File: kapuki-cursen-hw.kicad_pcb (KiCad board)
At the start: 2 copper layers, 27 parts, among them J1 Conn_01x02, J2 Conn_01x02, J3 Conn_01x01, J4 Conn_01x01, J5 Conn_01x01, J6 Conn_01x01, J7 Conn_01x06, J8 Conn_01x05, U1 MIC5235, U2 MAX4081S, U3 STM32G431KBUx

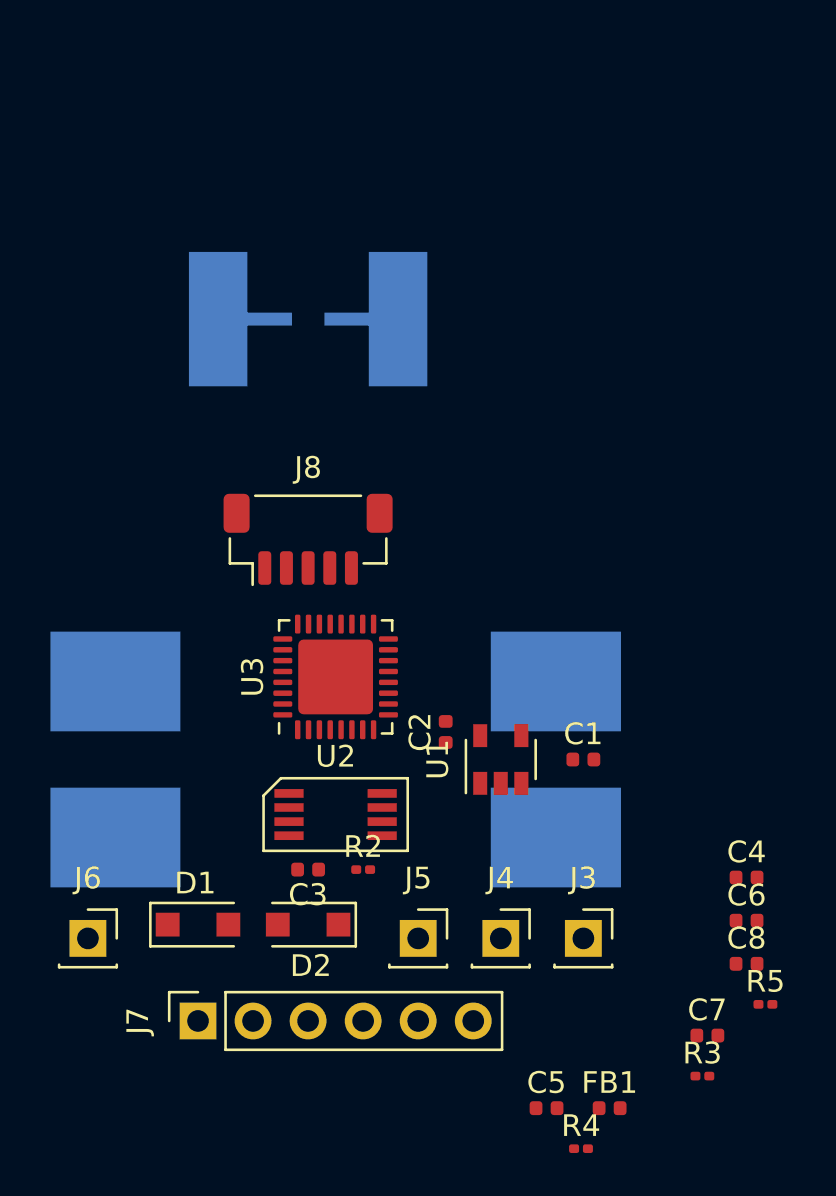
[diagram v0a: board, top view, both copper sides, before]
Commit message: Routing rev.1
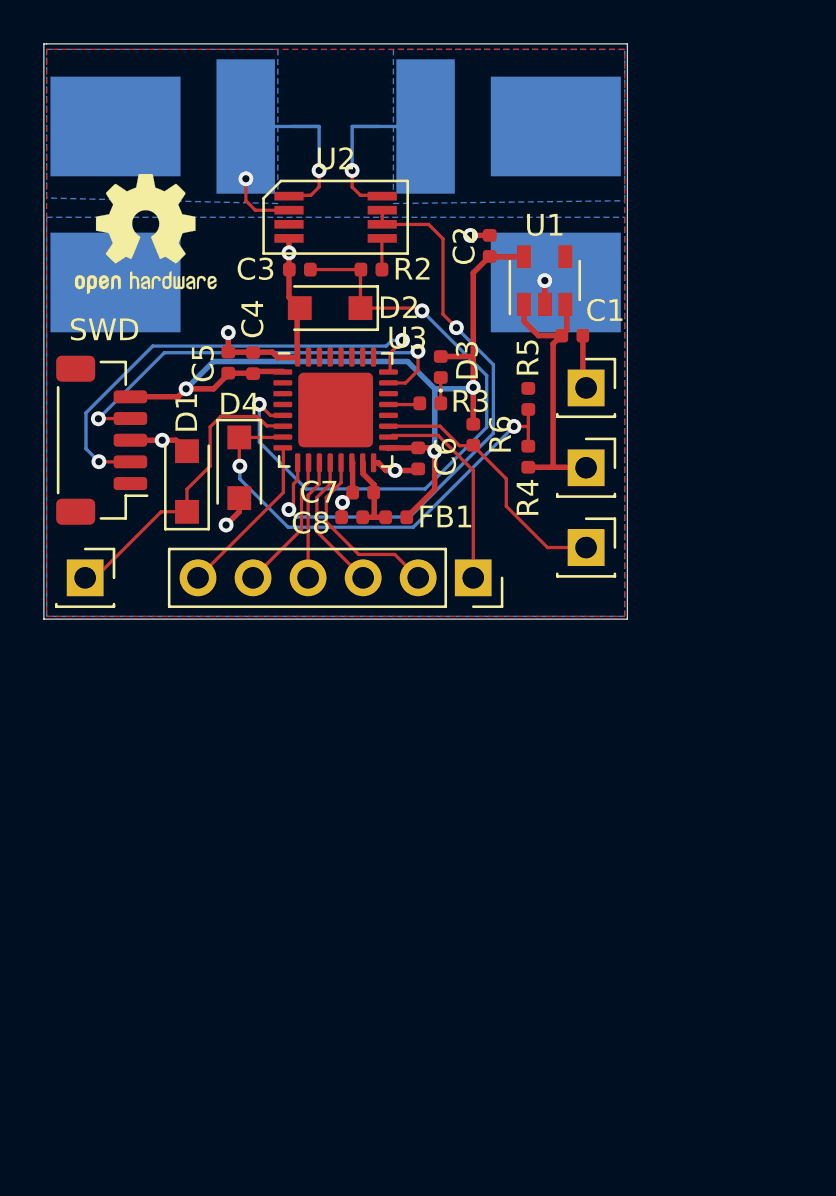
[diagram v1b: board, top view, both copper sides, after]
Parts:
- removed the R5 at (154.5, 91.3)
- added D3: LED, LED_SMD:LED_0402_1005Metric, F.Cu at (139.5, 61.9)
- added D4: BZT52H-C3V3, Diode_SMD:D_SOD-123F, F.Cu at (130.2, 66.5)
- added R3: R, Resistor_SMD:R_0402_1005Metric, F.Cu at (139.0, 63.6)
- added R6: R, Resistor_SMD:R_0402_1005Metric, F.Cu at (141.0, 65.0)
- added REF**: OSHW-Logo2_7.3x6mm_SilkScreen, Symbol:OSHW-Logo2_7.3x6mm_SilkScreen, F.Cu at (125.9, 55.8)
- R2: footprint Resistor_SMD:R_0201_0603Metric -> Resistor_SMD:R_0402_1005Metric
- R4: renamed from R3; footprint Resistor_SMD:R_0201_0603Metric -> Resistor_SMD:R_0402_1005Metric
- R5: renamed from R4; footprint Resistor_SMD:R_0201_0603Metric -> Resistor_SMD:R_0402_1005Metric
- moved C5 37.4 mm to (129.7, 61.7), turned to 90 degrees
- moved R5 34.7 mm to (143.5, 63.4), turned to 270 degrees
- moved C4 32.9 mm to (130.8, 61.7), turned to 90 degrees
- moved R4 29.7 mm to (143.5, 66.0), turned to 270 degrees
- moved C7 29.7 mm to (135.9, 67.7), turned to 180 degrees
- moved FB1 29.0 mm to (137.4, 68.8)
- moved D2 28.5 mm to (134.4, 59.2)
- moved C3 27.7 mm to (133.0, 57.4)
- moved R2 27.7 mm to (136.3, 57.4)
- moved U2 27.6 mm to (134.6, 55.0)
- moved C8 27.5 mm to (135.4, 68.8), turned to 180 degrees
- moved J5 26.6 mm to (146.2, 62.9)
- moved C6 26.2 mm to (138.4, 66.1), turned to 270 degrees
- moved J1 25.6 mm to (124.5, 54.4), turned to 0 degrees
- moved J2 25.6 mm to (144.8, 54.4), turned to 0 degrees
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- renumbered J3 to Je
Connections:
- net /VCC renamed VCC
- C7 pad 1: Net-(C7-Pad1) -> /VCCA
- C8 pad 1: Net-(C7-Pad1) -> /VCCA
- FB1 pad 1: Net-(C7-Pad1) -> /VCCA
- R1 pad 3: (no net) -> Net-(R1-Pad3)
- R1 pad 4: (no net) -> Net-(J2-Pad2)
- U3 pad 15: Net-(U3-Pad15) -> /VCCA
- U3 pad 21: Net-(U3-Pad21) -> /LED
- U3 pad 23: Net-(U3-Pad23) -> /SWCLK
- U3 pad 24: /SWCLK -> /SWDIO
- U3 pad 25: /SWDIO -> Net-(U3-Pad25)
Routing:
- net VCC: track 0.00 -> 41.7 mm, vias 0 -> 3
- net /CURRMEAS: track 0.00 -> 29.3 mm, vias 0 -> 2
- net /VREF: track 0.00 -> 27.1 mm, vias 0 -> 2
- net GND: track 0.00 -> 23.6 mm, vias 0 -> 8
- net Net-(D4-Pad1): track 0.00 -> 21.8 mm, vias 0 -> 2
- net /SWDIO: track 0.00 -> 21.6 mm, vias 0 -> 2
- net /SWCLK: track 0.00 -> 20.0 mm, vias 0 -> 2
- net /MOTORPULSE: track 0.00 -> 14.9 mm
- net /VCCIN: track 0.00 -> 13.2 mm
- net /RXTX: track 0.00 -> 12.1 mm
- net /EXT6: track 0.00 -> 9.47 mm
- net /EXT5: track 0.00 -> 8.35 mm
- net /EXT1: track 0.00 -> 7.60 mm
- net /EXT2: track 0.00 -> 6.39 mm
- net /EXT4: track 0.00 -> 6.34 mm
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- added copper zone on B.Cu, net GND
- added copper zone on F.Cu, net GND
- added copper zone on B.Cu, net Net-(J1-Pad2)
- added copper zone on B.Cu, net Net-(J2-Pad2)
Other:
- board outline added: 26.9 x 26.5 mm
- net class Default: clearance 0.2 -> 0.1524; trace_width 0.25 -> 0.1524; via_dia 0.8 -> 0.6858; via_drill 0.4 -> 0.3302
- net class VCC added: clearance 0.2032, trace_width 0.254, via_dia 0.6858, via_drill 0.3302
- rule pad_to_mask_clearance: 0.051 -> 0.0508
- rule solder_mask_min_width: 0.25 -> 0.0508
- rule trace_clearance: 0.2 -> 0.1524
- rule trace_min: 0.2 -> 0.1524
- rule via_min_drill: 0.3 -> 0.3302
- rule via_min_size: 0.4 -> 0.6858
- board text added: "SWD"
